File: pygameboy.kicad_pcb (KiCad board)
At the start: 2 copper layers, 49.3 x 59.7 mm, 79 parts, among them J1 Conn_01x01, J2 Conn_01x01, J3 Conn_ARM_JTAG_SWD_10, J4 USB_B_Micro, Q1 BSS138, U1 CARTRIDGE, U2 SAMD51J, U3 74LS244, U4 74LS244, U5 74x4245, U6 74LS244, U7 AP2204K-3.3

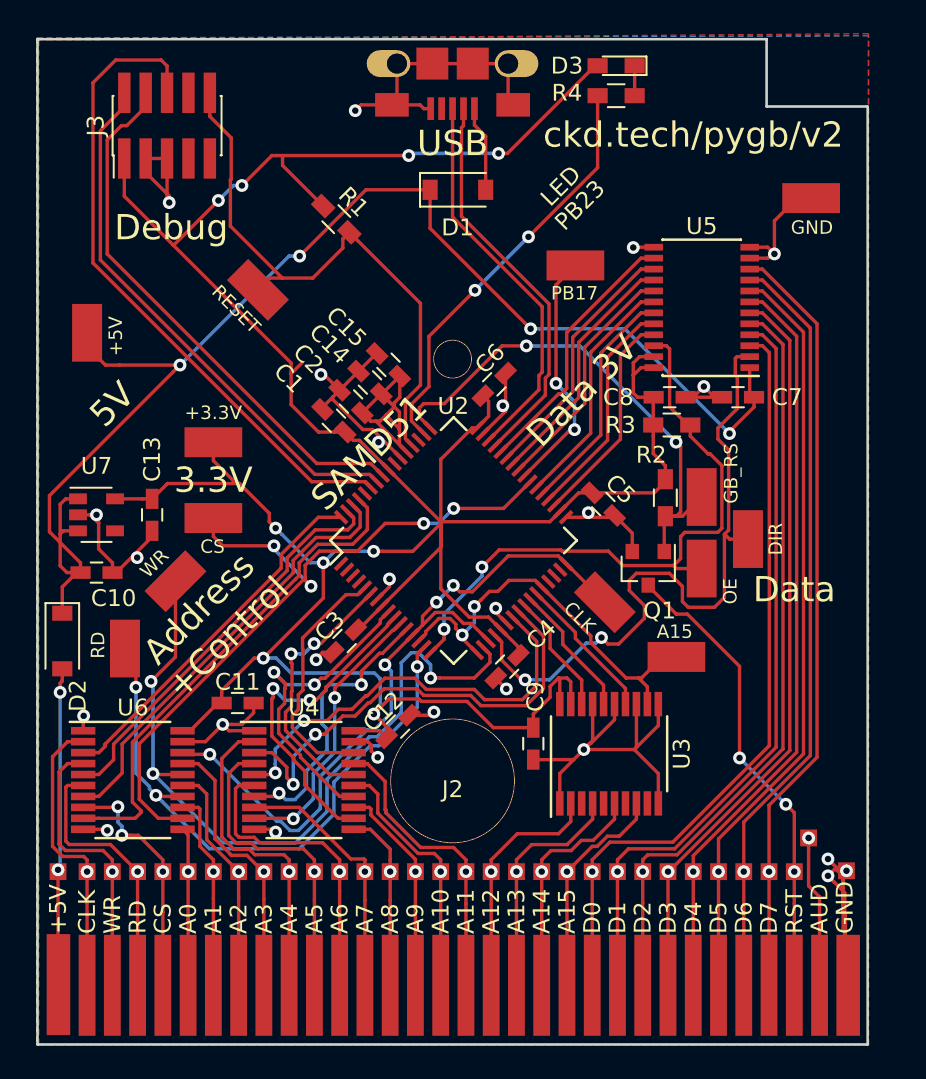
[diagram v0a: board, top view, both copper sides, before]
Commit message: v3
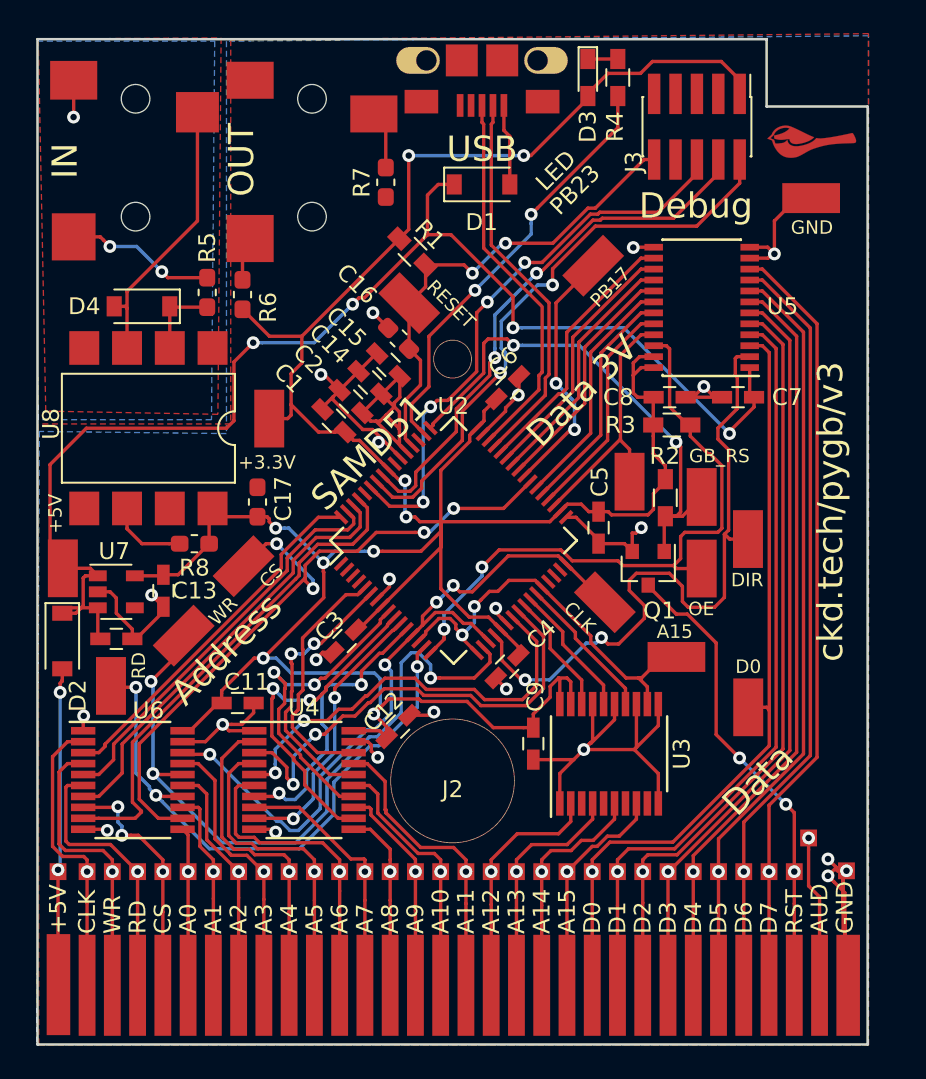
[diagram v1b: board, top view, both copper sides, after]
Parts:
- added C16: C_Small, Capacitor_SMD:C_0603_1608Metric_Pad1.05x0.95mm_HandSolder, F.Cu at (121.4, 56.1)
- added C17: C_Small, Capacitor_SMD:C_0603_1608Metric_Pad1.05x0.95mm_HandSolder, F.Cu at (113.1, 65.8)
- added D4: 1N4148W, Diode_SMD:D_SOD-123, F.Cu at (106.2, 54.2)
- added G***: LOGO, chickadee:chickadee_2mm_fcu, F.Cu at (146.0, 44.4)
- added J5: MIDI IN, cui-audio:CUI_SJ-3523-SMT-TR, F.Cu at (105.8, 45.3)
- added J6: MIDI OUT, cui-audio:CUI_SJ-3523-SMT-TR, F.Cu at (116.3, 45.3)
- added R5: R_Small, Resistor_SMD:R_0603_1608Metric_Pad1.05x0.95mm_HandSolder, F.Cu at (110.1, 53.3)
- added R6: R_Small, Resistor_SMD:R_0603_1608Metric_Pad1.05x0.95mm_HandSolder, F.Cu at (112.2, 53.5)
- added R7: R_Small, Resistor_SMD:R_0603_1608Metric_Pad1.05x0.95mm_HandSolder, F.Cu at (120.7, 46.8)
- added R8: 10k, Resistor_SMD:R_0603_1608Metric_Pad1.05x0.95mm_HandSolder, F.Cu at (109.3, 68.3)
- added TP46: data0, keystone:5015-SMT-TestPoint, F.Cu at (135.2, 64.6)
- added TP47: D0, keystone:5015-SMT-TestPoint, F.Cu at (142.2, 78.0)
- added U8: 6N137S, Package_DIP:SMDIP-8_W9.53mm, F.Cu at (106.6, 61.4)
- moved J3 31.5 mm to (139.2, 43.5), turned to 270 degrees
- moved TP39 14.1 mm to (101.5, 69.7)
- moved TP36 9.02 mm to (122.1, 54.0)
- moved R1 4.92 mm to (122.3, 50.9)
- moved U7 4.72 mm to (104.7, 71.1)
- moved C13 4.56 mm to (107.5, 71.1)
- moved C10 4.11 mm to (104.7, 73.9)
- moved TP38 3.60 mm to (113.8, 60.8), turned to 270 degrees
- moved TP45 3.37 mm to (112.2, 69.6), turned to 45 degrees
- moved TP42 3.27 mm to (108.7, 73.7)
- moved TP41 2.37 mm to (104.4, 76.7)
- moved D3 1.82 mm to (132.7, 40.6), turned to 270 degrees
- moved J4 1.76 mm to (126.4, 39.6)
- moved D1 1.47 mm to (126.4, 46.9)
- moved C5 1.43 mm to (133.3, 67.3), turned to 90 degrees
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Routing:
- net GND: track 133.6 -> 110.9 mm, vias 25 -> 23
- net Net-(D4-Pad2): track 0.00 -> 16.5 mm
- net Net-(J5-PadT): track 0.00 -> 8.93 mm, vias 0 -> 2
- net +3V3: track 190.4 -> 184.0 mm
- net /SAMD_RESET: track 35.0 -> 28.6 mm, vias 0 -> 2
- net /SWO: track 39.4 -> 34.0 mm, vias 0 -> 4
- net Net-(D4-Pad1): track 0.00 -> 4.72 mm
- net /MIDI_IN: track 0.00 -> 4.70 mm
- net Net-(J6-PadR): track 0.00 -> 3.58 mm
- net /3V_WR: track 45.6 -> 42.6 mm
- net /3V_D0: track 13.0 -> 15.8 mm
- net Net-(J6-PadT): track 0.00 -> 2.64 mm
- net +5V: track 82.4 -> 79.8 mm
- net /SWDIO: track 32.4 -> 34.9 mm, vias 0 -> 2
- net /SHIELD: track 0.00 -> 2.19 mm, vias 0 -> 1
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- added copper zone on B.Cu, net /SHIELD
- added copper zone on F.Cu, net /SHIELD
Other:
- board text added: "Address"
- board text added: "IN"
- board text added: "OUT"
- board text added: "ckd.tech/pygb/v3"
- board text removed: "3.3V"
- board text removed: "5V"
- board text removed: "Address +Control"
- board text removed: "ckd.tech/pygb/v2"
